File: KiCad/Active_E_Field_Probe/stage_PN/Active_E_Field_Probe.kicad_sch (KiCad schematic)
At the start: 14 parts

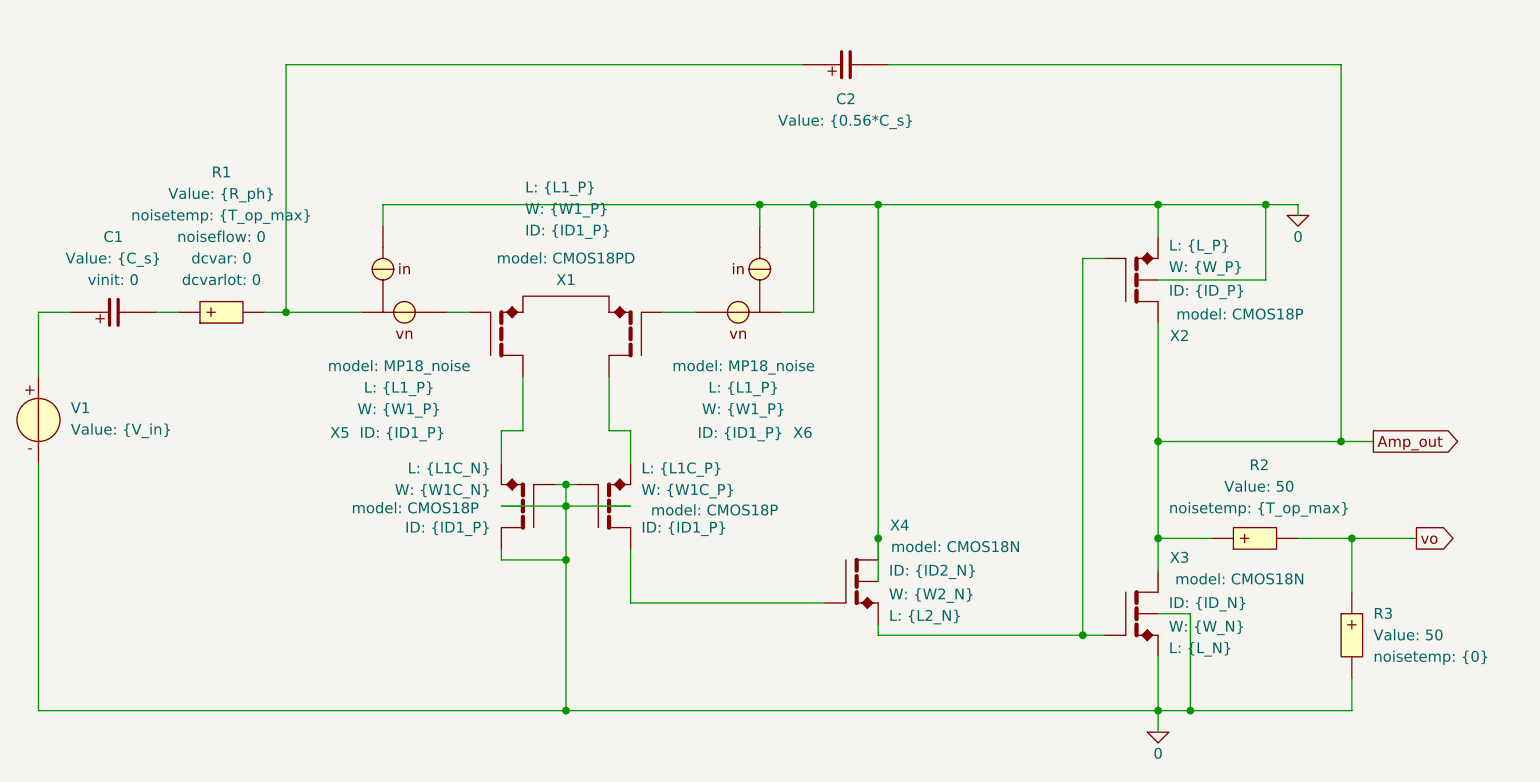
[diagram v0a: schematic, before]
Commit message: diff vf
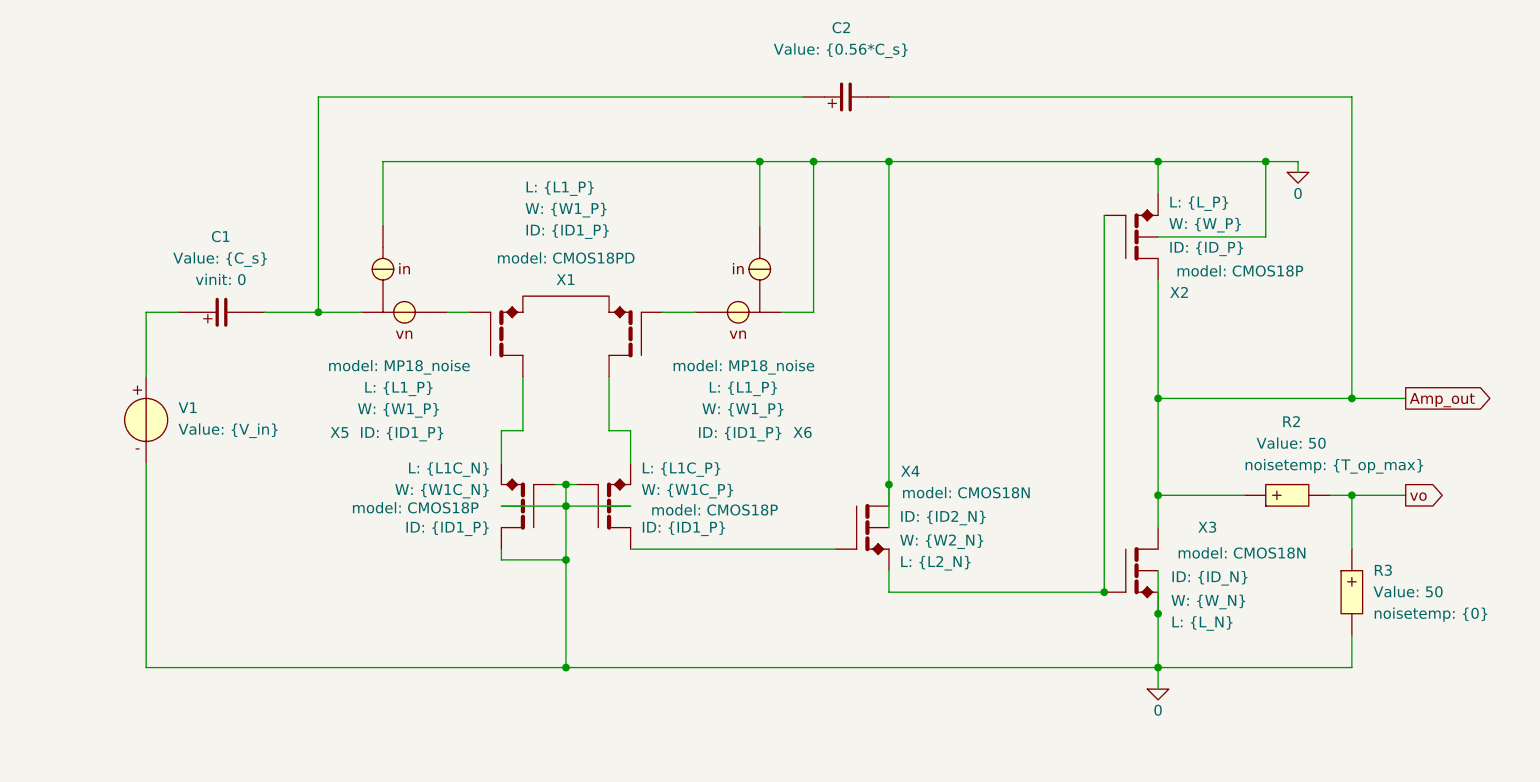
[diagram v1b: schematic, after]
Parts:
- removed R1: {R_ph}, symbol SLiCAP:R
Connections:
- net at C2.1, X5.1 (ext): now also C1.2
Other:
- moved on the sheet: C1, C2, R2, R3, V1, X2, X3, X4
